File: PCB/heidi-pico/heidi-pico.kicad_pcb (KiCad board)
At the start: 2 copper layers, 21 x 51 mm, 32 parts, among them J1 USB_C_Receptacle_USB2.0_14P, J2 Conn_01x03, J3 Conn_01x20, J4 Conn_01x20, SW1 SW_Push, U1 RP2040, U2 MCP1700x-330xxTT, U3 W25Q16JVZPIQ TR, Y1 ABM8-272-T3

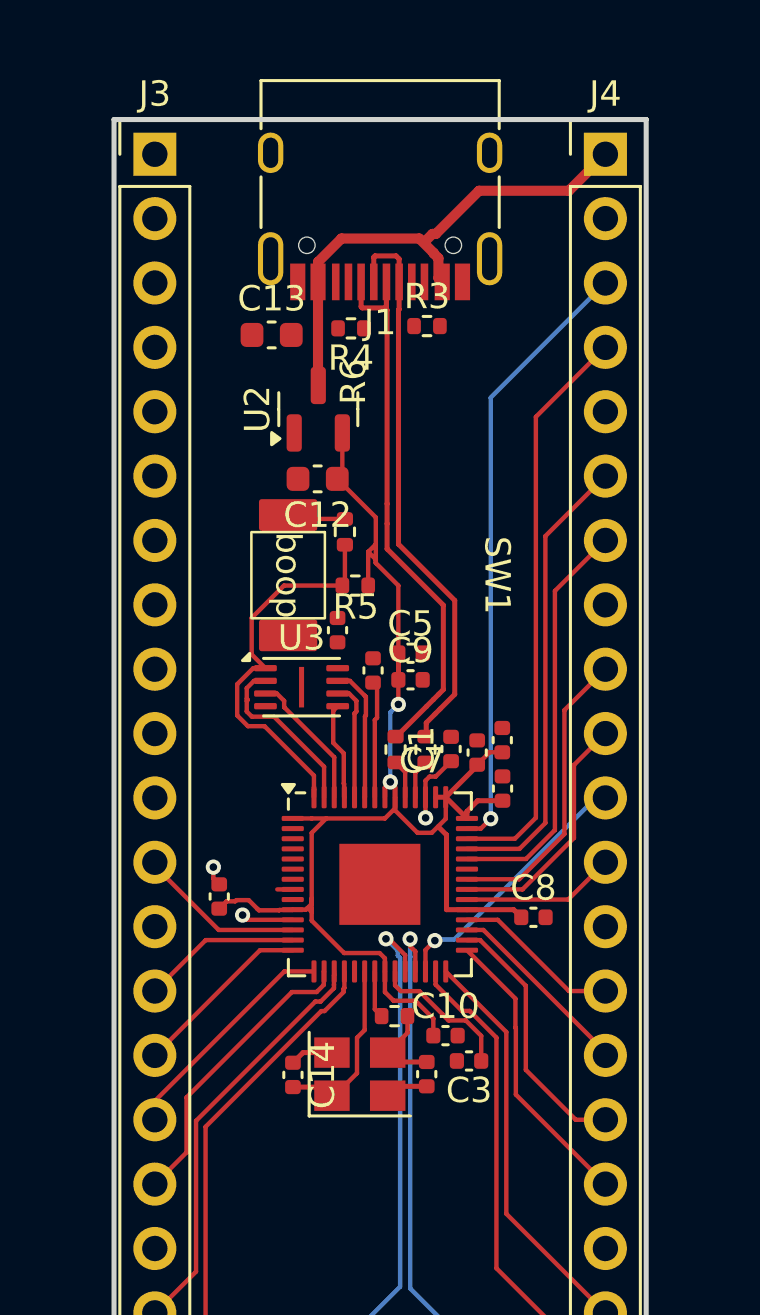
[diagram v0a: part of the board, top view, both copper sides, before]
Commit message: AHHHH ROUTING
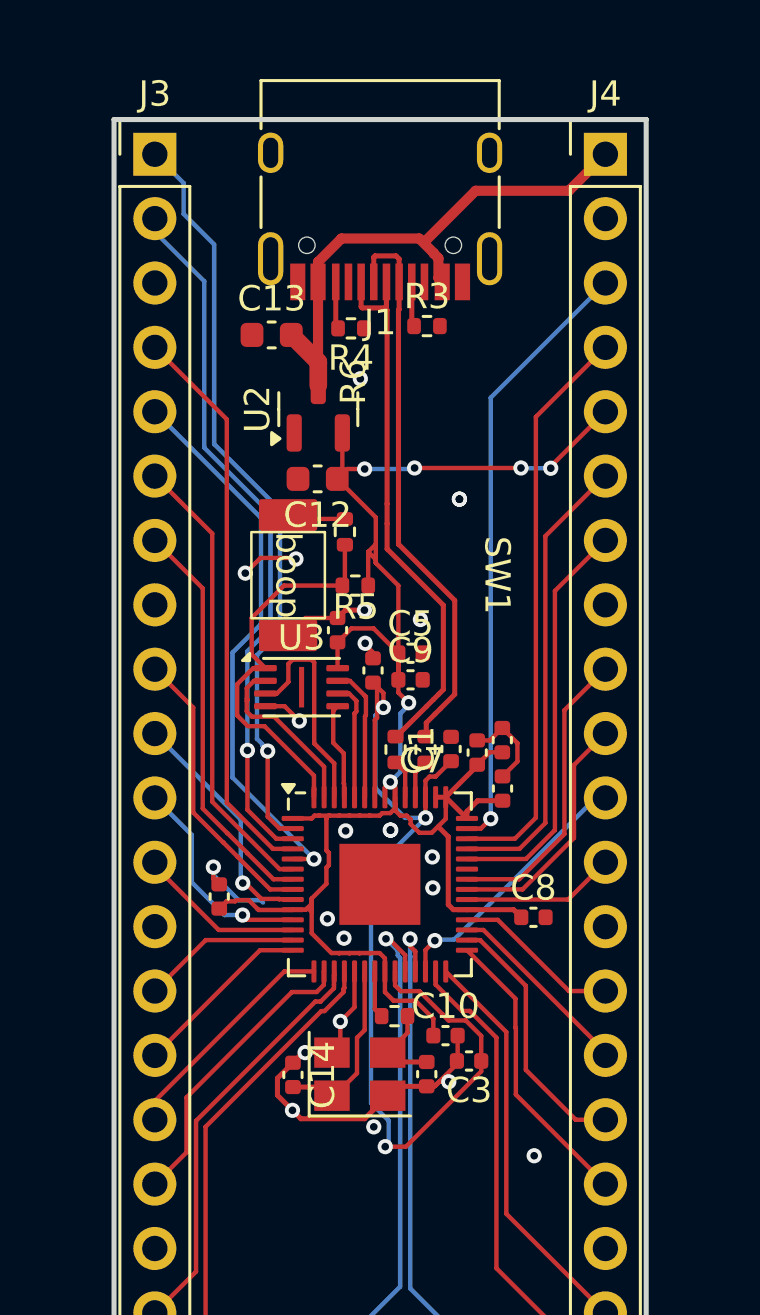
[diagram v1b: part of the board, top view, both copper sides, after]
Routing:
- net GPIO0: track 0.00 -> 29.9 mm, vias 0 -> 1
- net GPIO1: track 0.00 -> 27.9 mm, vias 0 -> 1
- net GND: track 4.17 -> 32.0 mm, vias 1 -> 23
- net +1V1: track 13.2 -> 39.9 mm, vias 1 -> 3
- net GPIO2: track 0.00 -> 22.5 mm
- net GPIO3: track 0.00 -> 22.2 mm, vias 0 -> 1
- net GPIO4: track 0.00 -> 18.1 mm
- net +3V3: track 58.4 -> 75.0 mm, vias 2 -> 6
- net GPIO5: track 0.00 -> 16.1 mm
- net GPIO6: track 0.61 -> 11.5 mm
- net GPIO7: track 0.00 -> 9.58 mm, vias 0 -> 1
- net GPIO8: track 2.06 -> 8.53 mm
- net QSPI_SD2: track 5.48 -> 8.59 mm
- net VBUS: track 19.4 -> 21.8 mm
- net Net-(J1-CC2): track 0.00 -> 1.87 mm
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
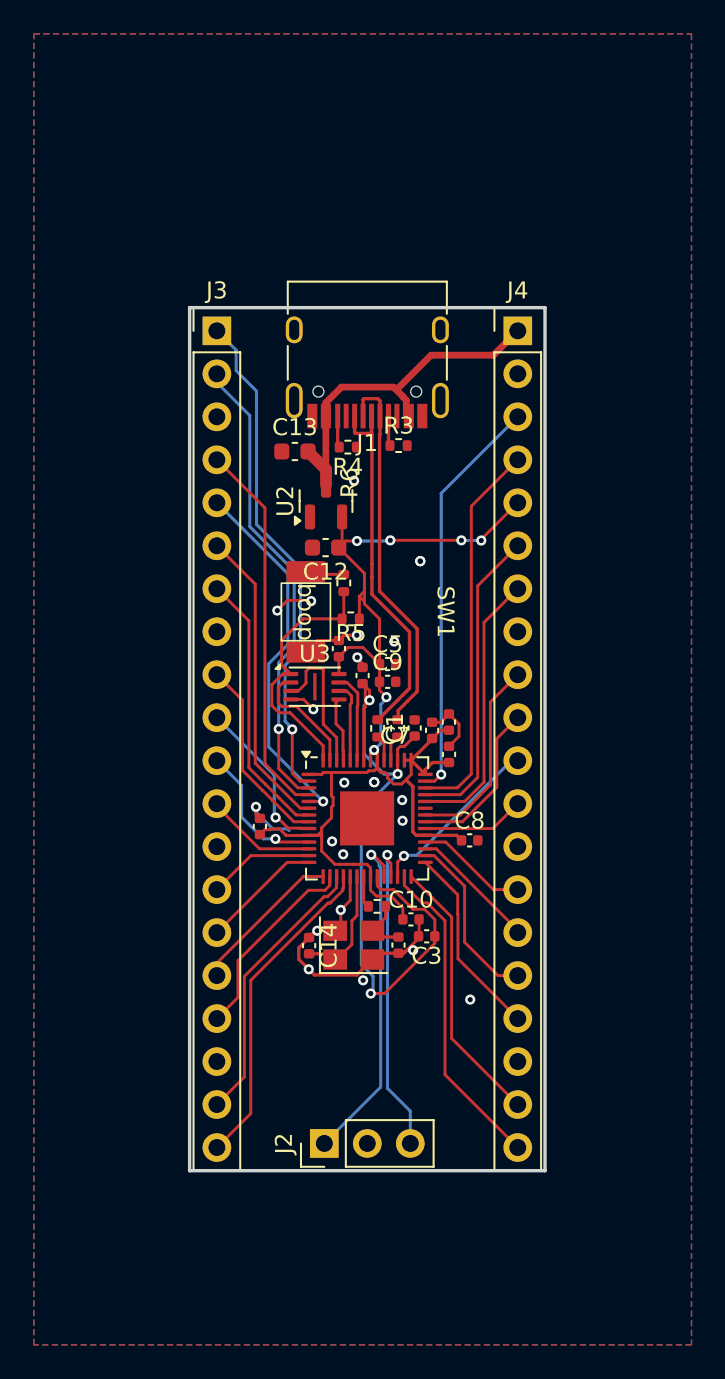
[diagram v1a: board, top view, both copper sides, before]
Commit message: LCSC BOM
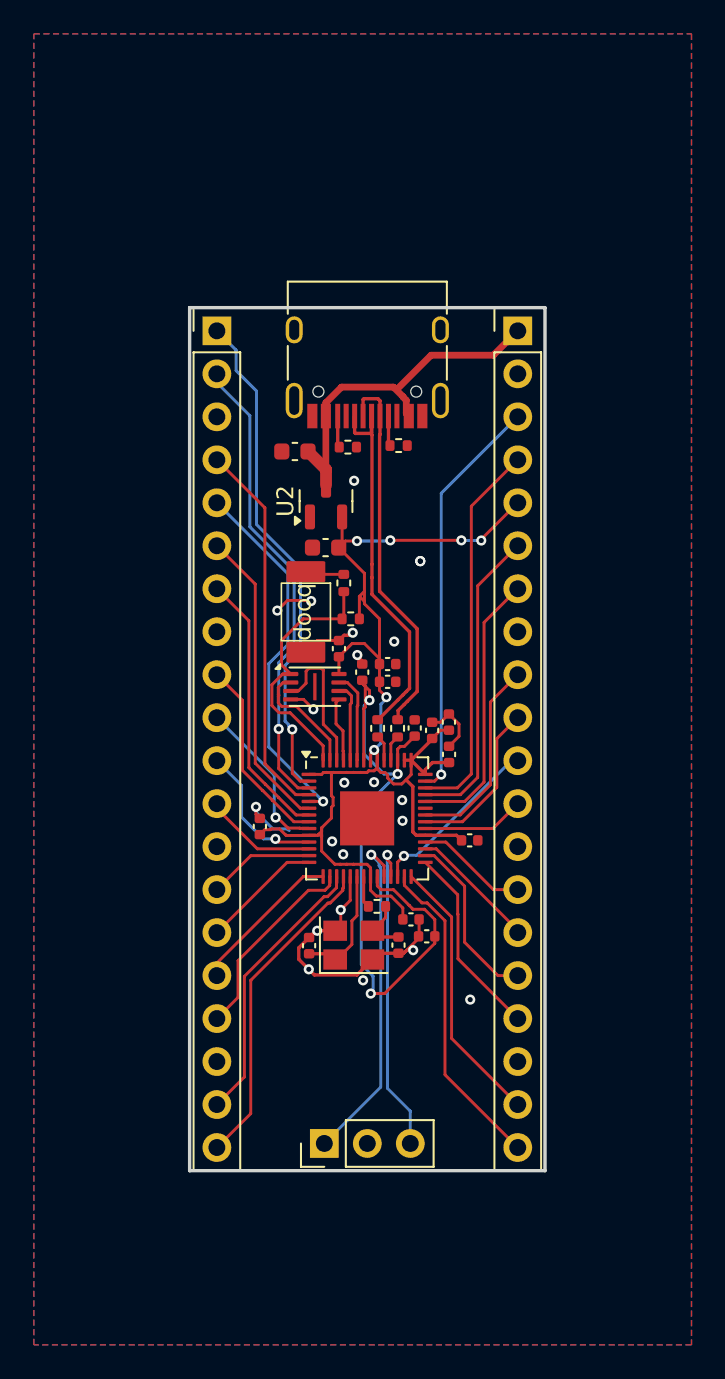
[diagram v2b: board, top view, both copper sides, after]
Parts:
- moved C2 0.20 mm to (92.0, 96.1)
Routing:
- net GND: track 32.0 -> 31.9 mm, vias 23 -> 22
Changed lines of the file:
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@@
 			(outputformat 1)
 			(mirror no)
-			(drillshape 1)
+			(drillshape 0)
 			(scaleselection 1)
-			(outputdirectory "")
+			(outputdirectory "C:/Users/willi/Desktop/hc/gtihub clone/heidi-pico/PCB/heidi-pico/GERBERS/try1/")
 		)
 	)
@@
 			(at 0 -1.95 0)
 			(layer "F.SilkS")
+			(hide yes)
 			(effects
 				(font
@@
 			(at 0 -1.16 0)
 			(layer "F.SilkS")
+			(hide yes)
 			(effects
 				(font
@@
 		)
 		(property "Value" "100n"
-			(at 0 1.16 0)
+			(at 0 1.02 0)
 			(layer "F.Fab")
 			(effects
@@
 			(at 0 -1.16 0)
 			(layer "F.SilkS")
+			(hide yes)
 			(effects
 				(font
@@
 			(at 0 -2.38 0)
 			(layer "F.SilkS")
+			(hide yes)
 			(effects
 				(font
@@
 			(at -5.93 -0.3325 90)
 			(layer "F.SilkS")
+			(hide yes)
 			(effects
 				(font
@@
 			(at 0 -2.38 90)
 			(layer "F.SilkS")
+			(hide yes)
 			(effects
 				(font
@@
 		(tags "capacitor")
 		(property "Reference" "C7"
-			(at 1.096361 -3.174076 0)
+			(at 1.3 -3.79 0)
 			(layer "F.SilkS")
+			(hide yes)
 			(effects
 				(font
@@
 			(at 0 -1.16 0)
 			(layer "F.SilkS")
+			(hide yes)
 			(effects
 				(font
@@
 			(at 0 -5.645 180)
 			(layer "F.SilkS")
+			(hide yes)
 			(effects
 				(font
@@
 			(unlocked yes)
 			(layer "F.SilkS")
+			(hide yes)
 			(effects
 				(font
@@
 			(at -0.02 -0.8425 0)
 			(layer "F.SilkS")
+			(hide yes)
 			(effects
 				(font
@@
 			(at 0 -1.17 0)
 			(layer "F.SilkS")
+			(hide yes)
 			(effects
 				(font
@@
 			(at 0 -1.16 0)
 			(layer "F.SilkS")
+			(hide yes)
 			(effects
 				(font
@@
 			(at 0 -1.16 90)
 			(layer "F.SilkS")
+			(hide yes)
 			(effects
 				(font
@@
 			(at 0 -1.17 0)
 			(layer "F.SilkS")
+			(hide yes)
 			(effects
 				(font
@@
 		(tags "capacitor")
 		(property "Reference" "C14"
-			(at 0 -1.16 90)
+			(at 0.13 -1.53 90)
 			(layer "F.SilkS")
+			(hide yes)
 			(effects
 				(font
@@
 			(at 0 -2.38 0)
 			(layer "F.SilkS")
+			(hide yes)
 			(effects
 				(font
@@
 	(footprint "Capacitor_SMD:C_0402_1005Metric"
 		(layer "F.Cu")
-		(at 92.07 96.34 90)
+		(at 92.05 96.14 90)
 		(descr "Capacitor SMD 0402 (1005 Metric), square (rectangular) end terminal, IPC-7351 nominal, (Body size source: IPC-SM-782 page 76, https://www.pcb-3d.com/wordpress/wp-content/uploads/ipc-sm-782a_amendment_1_and_2.pdf), generated with kicad-footprint-generator")
 		(tags "capacitor")
@@
 		)
 		(property "Value" "100n"
-			(at 0 1.16 90)
+			(at 0.14 1.16 90)
 			(layer "F.Fab")
 			(effects
@@
 			(at 0 -1.43 0)
 			(layer "F.SilkS")
+			(hide yes)
 			(effects
 				(font
@@
 			(at 0 -1.16 0)
 			(layer "F.SilkS")
+			(hide yes)
 			(effects
 				(font
@@
 			(at 0 -1.43 0)
 			(layer "F.SilkS")
+			(hide yes)
 			(effects
 				(font
@@
 	)
 	(segment
+		(start 91.34 93.96)
+		(end 90.98 93.96)
+		(width 0.2)
+		(layer "F.Cu")
+		(net 1)
+	)
+	(segment
 		(start 95.41 111.72)
 		(end 95.38 111.75)
@@
 	)
 	(segment
-		(start 91.76 95.34)
-		(end 92.07 95.65)
+		(start 91.76 95.2)
+		(end 92.07 95.51)
 		(width 0.2)
 		(layer "F.Cu")
@@
 	)
 	(segment
-		(start 91.73 93.96)
-		(end 90.98 93.96)
-		(width 0.2)
+		(start 89.02 91.9)
+		(end 87.63 91.9)
+		(width 0.175)
 		(layer "F.Cu")
 		(net 1)
 	)
 	(segment
-		(start 89.02 91.9)
-		(end 87.63 91.9)
-		(width 0.175)
+		(start 90.98 93.96)
+		(end 90.67 94.27)
+		(width 0.2)
 		(layer "F.Cu")
 		(net 1)
@@
 	)
 	(segment
-		(start 90.98 93.96)
-		(end 90.67 94.27)
-		(width 0.2)
-		(layer "F.Cu")
-		(net 1)
-	)
-	(segment
 		(start 95.38 111.87)
 		(end 94.5 112.75)
@@
 	)
 	(segment
-		(start 92.07 95.65)
-		(end 92.07 95.86)
+		(start 92.07 95.51)
+		(end 92.07 95.72)
 		(width 0.2)
 		(layer "F.Cu")
@@
 	)
 	(segment
+		(start 91.49 93.81)
+		(end 91.34 93.96)
+		(width 0.2)
+		(layer "F.Cu")
+		(net 1)
+	)
+	(segment
 		(start 95.06 112.57)
 		(end 94.68 112.57)
@@
 	)
 	(via
-		(at 91.73 93.96)
+		(at 91.49 93.81)
 		(size 0.6)
 		(drill 0.3)
@@
 	)
 	(via
-		(at 91.76 95.2675)
+		(at 91.76 95.1275)
 		(size 0.6)
 		(drill 0.3)
@@
 	)
 	(via
-		(at 92.77 102.64)
-		(size 0.6)
-		(drill 0.3)
-		(layers "F.Cu" "B.Cu")
-		(free yes)
-		(net 1)
-	)
-	(via
 		(at 95.48 89.58)
 		(size 0.6)
@@
 	)
 	(segment
-		(start 91.22 94.68)
-		(end 90.67 95.23)
-		(width 0.175)
-		(layer "F.Cu")
-		(net 3)
-	)
-	(segment
 		(start 96.32 99.91)
 		(end 96.32 99.9625)
@@
 	)
 	(segment
-		(start 93.07 95.66)
-		(end 92.09 94.68)
-		(width 0.175)
-		(layer "F.Cu")
-		(net 3)
-	)
-	(segment
 		(start 92.9515 101.6215)
 		(end 92.9515 101.871598)
@@
 	)
 	(segment
+		(start 92.18 94.45)
+		(end 91.45 94.45)
+		(width 0.175)
+		(layer "F.Cu")
+		(net 3)
+	)
+	(segment
 		(start 91.531598 107.4915)
 		(end 91.54 107.499902)
@@
 	)
 	(segment
-		(start 92.09 94.68)
-		(end 91.22 94.68)
-		(width 0.175)
-		(layer "F.Cu")
-		(net 3)
-	)
-	(segment
 		(start 90.3285 103.536235)
 		(end 90.3285 104.023765)
@@
 	)
 	(segment
+		(start 93.07 95.66)
+		(end 93.07 95.34)
+		(width 0.175)
+		(layer "F.Cu")
+		(net 3)
+	)
+	(segment
 		(start 92.76 100.63)
 		(end 92.7525 100.6375)
@@
 	)
 	(segment
+		(start 91.45 94.45)
+		(end 90.67 95.23)
+		(width 0.175)
+		(layer "F.Cu")
+		(net 3)
+	)
+	(segment
 		(start 93.3985 102.0685)
 		(end 93.555192 102.225192)
@@
 	)
 	(segment
+		(start 93.07 95.34)
+		(end 92.18 94.45)
+		(width 0.175)
+		(layer "F.Cu")
+		(net 3)
+	)
+	(segment
 		(start 90.66 88.78)
 		(end 92.18 90.3)
@@
 	(segment
 		(start 88.9025 106.58)
-		(end 85.980128 106.58)
+		(end 85.85 106.58)
 		(width 0.175)
 		(layer "F.Cu")
@@
 	)
 	(segment
-		(start 85.980128 106.58)
-		(end 83.46 104.059872)
+		(start 83.46 104.19)
+		(end 83.46 103.91)
 		(width 0.175)
 		(layer "F.Cu")
@@
 	)
 	(segment
-		(start 83.46 104.059872)
-		(end 83.46 103.91)
+		(start 85.85 106.58)
+		(end 83.46 104.19)
 		(width 0.175)
 		(layer "F.Cu")
@@
 	)
 	(segment
-		(start 91.34 101.3425)
-		(end 91.34 98.033122)
+		(start 91.34 98.033122)
+		(end 91.4135 97.959622)
 		(width 0.175)
 		(layer "F.Cu")
@@
 	)
 	(segment
-		(start 91.4135 97.540378)
-		(end 91.123122 97.25)
+		(start 91.4135 97.959622)
+		(end 91.4135 97.540378)
 		(width 0.175)
 		(layer "F.Cu")
@@
 	)
 	(segment
-		(start 91.4135 97.959622)
-		(end 91.4135 97.540378)
+		(start 91.123122 97.25)
+		(end 90.675 97.25)
 		(width 0.175)
 		(layer "F.Cu")
@@
 	)
 	(segment
-		(start 91.34 98.033122)
-		(end 91.4135 97.959622)
+		(start 91.34 101.3425)
+		(end 91.34 98.033122)
 		(width 0.175)
 		(layer "F.Cu")
@@
 	)
 	(segment
-		(start 91.123122 97.25)
-		(end 90.675 97.25)
+		(start 91.4135 97.540378)
+		(end 91.123122 97.25)
 		(width 0.175)
 		(layer "F.Cu")
@@
 	)
 	(segment
-		(start 91.7515 97.346634)
-		(end 91.7515 97.344757)
+		(start 91.7895 97.3695)
+		(end 91.17 96.75)
 		(width 0.175)
 		(layer "F.Cu")
@@
 	)
 	(segment
-		(start 91.7515 101.331)
-		(end 91.7515 98.153366)
-		(width 0.175)
-		(layer "F.Cu")
-		(net 49)
-	)
-	(segment
-		(start 91.7515 97.344757)
-		(end 91.156743 96.75)
-		(width 0.175)
-		(layer "F.Cu")
-		(net 49)
-	)
-	(segment
-		(start 91.7895 98.115366)
-		(end 91.7895 97.384634)
+		(start 91.17 96.75)
+		(end 90.675 96.75)
 		(width 0.175)
 		(layer "F.Cu")
@@
 	)
 	(segment
-		(start 91.156743 96.75)
-		(end 90.675 96.75)
+		(start 91.74 101.3425)
+		(end 91.7515 101.331)
 		(width 0.175)
 		(layer "F.Cu")
@@
 	)
 	(segment
-		(start 91.74 101.3425)
-		(end 91.7515 101.331)
+		(start 91.7515 101.331)
+		(end 91.7515 98.153366)
 		(width 0.175)
 		(layer "F.Cu")
@@
 	)
 	(segment
-		(start 91.7895 97.384634)
-		(end 91.7515 97.346634)
+		(start 91.7895 98.115366)
+		(end 91.7895 97.3695)
 		(width 0.175)
 		(layer "F.Cu")
